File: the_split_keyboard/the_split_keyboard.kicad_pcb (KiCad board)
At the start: 2 copper layers, 1 part, among them U1 ProMicro_r

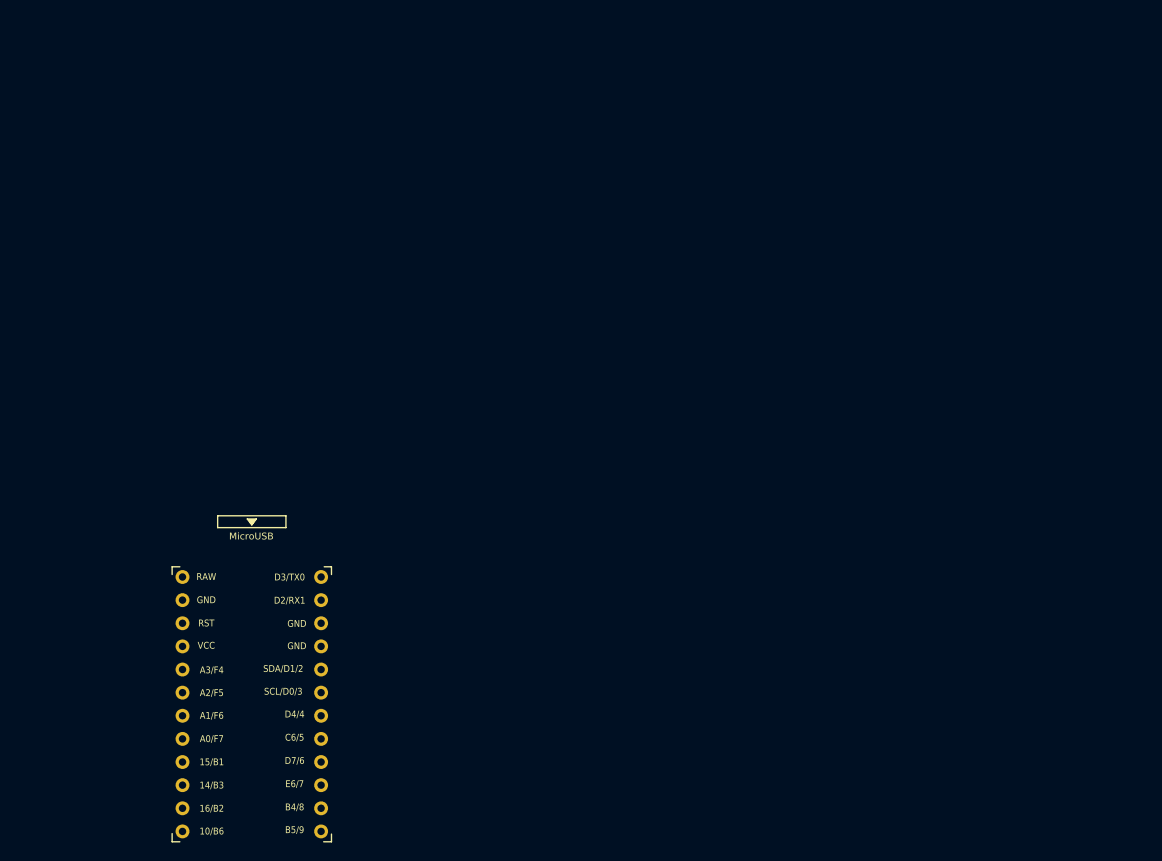
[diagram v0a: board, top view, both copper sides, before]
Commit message: 色々追加
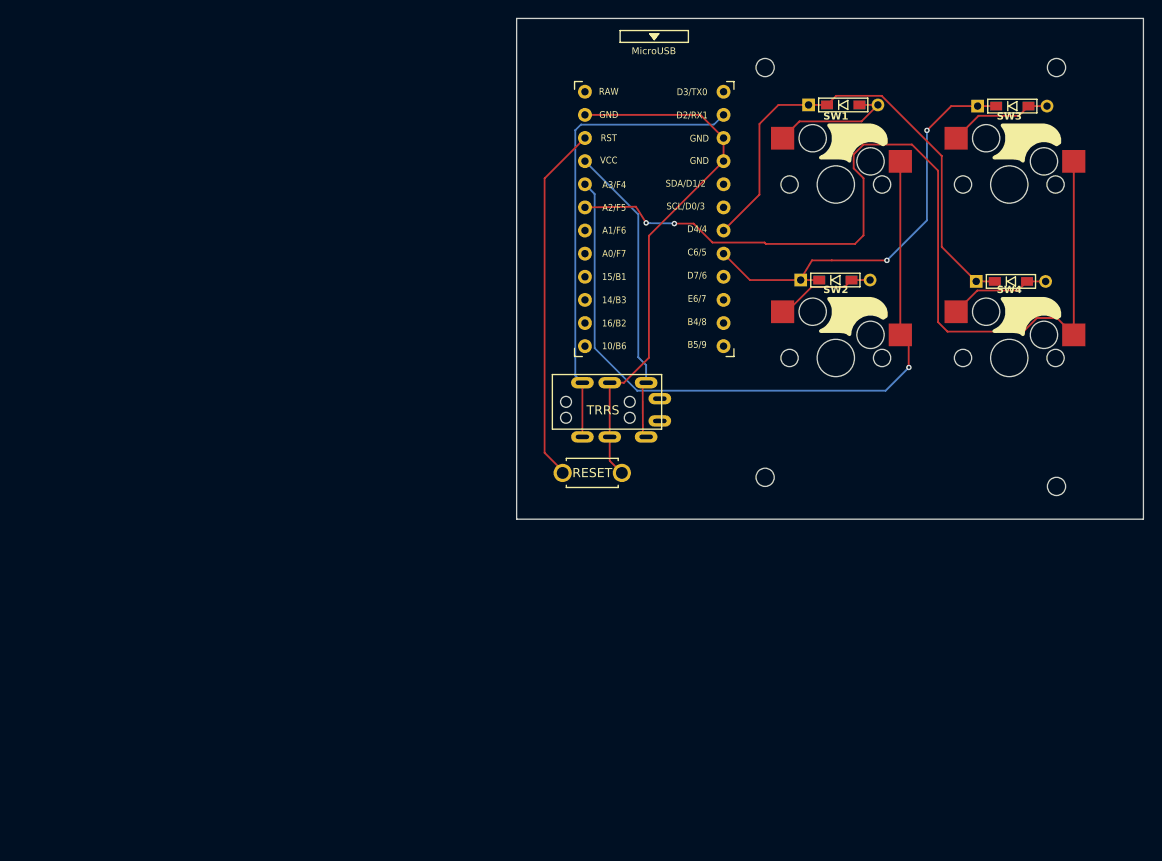
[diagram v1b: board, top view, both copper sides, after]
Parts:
- added D1: D, keyboard:D3_TH_SMD, F.Cu at (136.6, 40.1)
- added D2: D, keyboard:D3_TH_SMD, F.Cu at (135.7, 59.3)
- added D3: D, keyboard:D3_TH_SMD, F.Cu at (155.1, 40.2)
- added D4: D, keyboard:D3_TH_SMD, F.Cu at (155.0, 59.5)
- added J2: MJ-4PP-9, keyboard:MJ-4PP-9, F.Cu at (104.6, 72.7)
- added SW1: SW_PUSH, kbd:keyswitch_cherrymx_hotswap_1u, F.Cu at (135.8, 48.8)
- added SW2: SW_PUSH, kbd:keyswitch_cherrymx_hotswap_1u, F.Cu at (135.8, 67.9)
- added SW3: SW_PUSH, kbd:keyswitch_cherrymx_hotswap_1u, F.Cu at (154.8, 48.8)
- added SW4: SW_PUSH, kbd:keyswitch_cherrymx_hotswap_1u, F.Cu at (154.8, 67.9)
- added SW5: SW_PUSH, kbd:ResetSW, F.Cu at (109.0, 80.5)
- U1: value ProMicro_r -> ProMicro
- moved U1 69.2 mm to (115.8, 53.1)
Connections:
- U1 pad 1: (no net) -> unconnected-(U1-TX0/D3-Pad1)
- U1 pad 10: (no net) -> unconnected-(U1-7/E6-Pad10)
- U1 pad 11: (no net) -> unconnected-(U1-8/B4-Pad11)
- U1 pad 12: (no net) -> unconnected-(U1-9/B5-Pad12)
- U1 pad 13: (no net) -> unconnected-(U1-B6/10-Pad13)
- U1 pad 14: (no net) -> unconnected-(U1-B2/16-Pad14)
- U1 pad 15: (no net) -> unconnected-(U1-B3/14-Pad15)
- U1 pad 16: (no net) -> unconnected-(U1-B1/15-Pad16)
- U1 pad 17: (no net) -> unconnected-(U1-F7/A0-Pad17)
- U1 pad 18: (no net) -> unconnected-(U1-F6/A1-Pad18)
- U1 pad 19: (no net) -> col1
- U1 pad 2: (no net) -> data
- U1 pad 20: (no net) -> col0
- U1 pad 21: (no net) -> VCC
- U1 pad 22: (no net) -> reset
- U1 pad 23: (no net) -> GND
- U1 pad 24: (no net) -> unconnected-(U1-RAW-Pad24)
- U1 pad 3: (no net) -> GND
- U1 pad 4: (no net) -> GND
- U1 pad 5: (no net) -> unconnected-(U1-2/D1/SDA-Pad5)
- U1 pad 6: (no net) -> unconnected-(U1-3/D0/SCL-Pad6)
- U1 pad 7: (no net) -> row0
- U1 pad 8: (no net) -> row1
- U1 pad 9: (no net) -> unconnected-(U1-6/D7-Pad9)
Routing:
- net col1: track 0.00 -> 94.7 mm, vias 0 -> 2
- net col0: track 0.00 -> 75.0 mm, vias 0 -> 1
- net GND: track 0.00 -> 59.7 mm
- net row0: track 0.00 -> 54.8 mm
- net data: track 0.00 -> 51.0 mm
- net row1: track 0.00 -> 42.6 mm, vias 0 -> 2
- net reset: track 0.00 -> 39.4 mm
- net VCC: track 0.00 -> 27.1 mm
- net Net-(D1-A): track 0.00 -> 14.0 mm
- net Net-(D3-A): track 0.00 -> 11.4 mm
- net Net-(D4-A): track 0.00 -> 11.2 mm
- net Net-(D2-A): track 0.00 -> 11.0 mm
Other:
- board outline added: 68.8 x 55 mm

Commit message: update
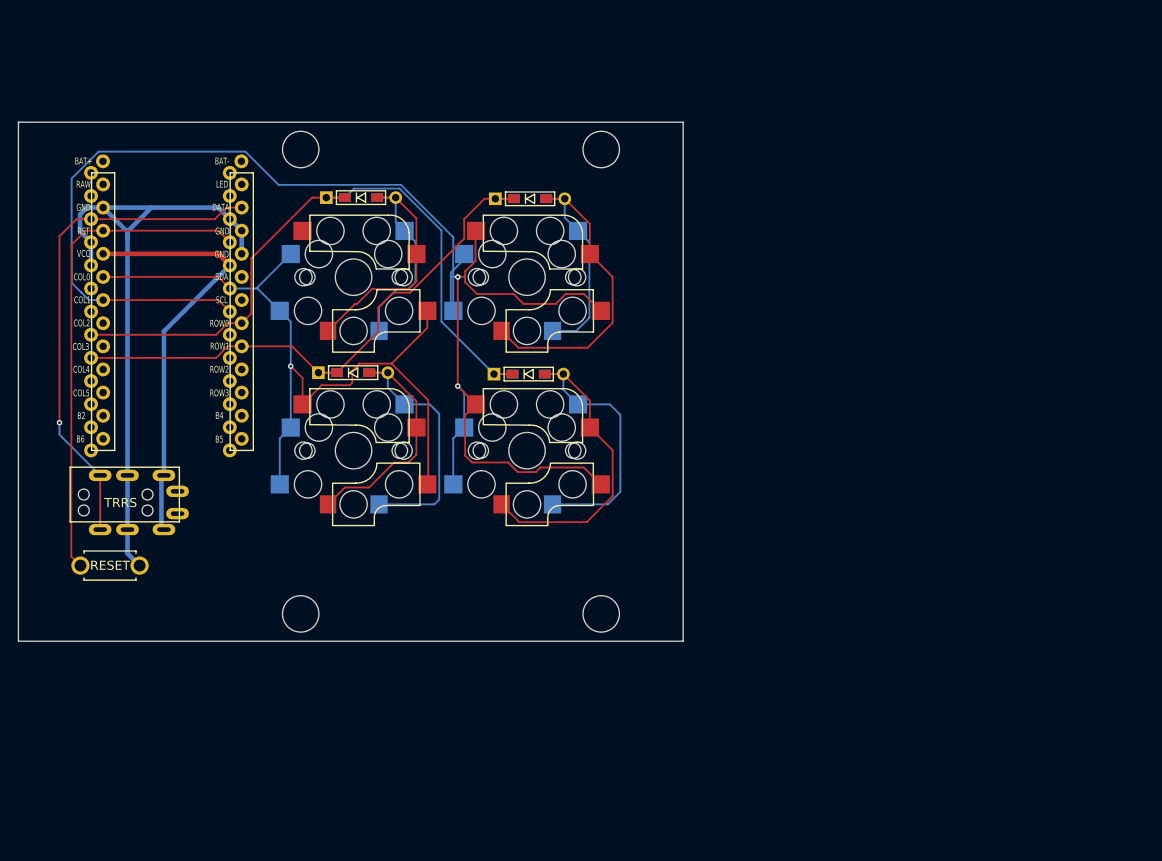
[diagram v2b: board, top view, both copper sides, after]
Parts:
- SW1, SW2, SW3, SW4: footprint kbd:keyswitch_cherrymx_hotswap_1u -> keyboard:MX_Choc_Hotswap
- U1: footprint kbd:ProMicro -> keyboard:ProMicro_v2
- moved D1 53.9 mm to (83.6, 50.3)
- moved D2 53.9 mm to (82.8, 69.5)
- moved SW1 53.9 mm to (82.8, 59.0)
- moved SW2 53.9 mm to (82.8, 78.1)
- moved SW5 53.9 mm to (56.1, 90.7)
- moved U1 53.9 mm to (62.9, 63.3)
- moved D3 53.9 mm to (102.2, 50.4)
- moved D4 53.9 mm to (102.0, 69.7)
- moved J2 53.9 mm to (51.7, 82.9)
- moved SW3 53.9 mm to (101.9, 59.0)
- moved SW4 53.9 mm to (101.9, 78.1)
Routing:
- net col1: track 94.7 -> 164.6 mm
- net Net-(D4-A): track 11.2 -> 59.5 mm
- net Net-(D3-A): track 11.4 -> 52.8 mm
- net Net-(D2-A): track 11.0 -> 51.0 mm
- net Net-(D1-A): track 14.0 -> 44.1 mm
- net row1: track 42.6 -> 62.9 mm, vias 2 -> 0
- net row0: track 54.8 -> 74.8 mm
- net VCC: track 27.1 -> 46.7 mm
- net reset: track 39.4 -> 54.2 mm
- net GND: track 59.7 -> 73.2 mm
- net col0: track 75.0 -> 85.8 mm
- net data: track 51.0 -> 55.4 mm, vias 0 -> 1
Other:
- board size 68.8 x 55 mm -> 73 x 57 mm
